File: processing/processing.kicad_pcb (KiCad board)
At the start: 2 copper layers, 26 parts, among them J1 HRO-TYPE-C-31-M-12, J2 Conn_01x03, J3 ICSP, SW1 SW_RESET, U1 CH340G, U2 ATmega328P-AU, Y1 12MHz, Y2 16MHz

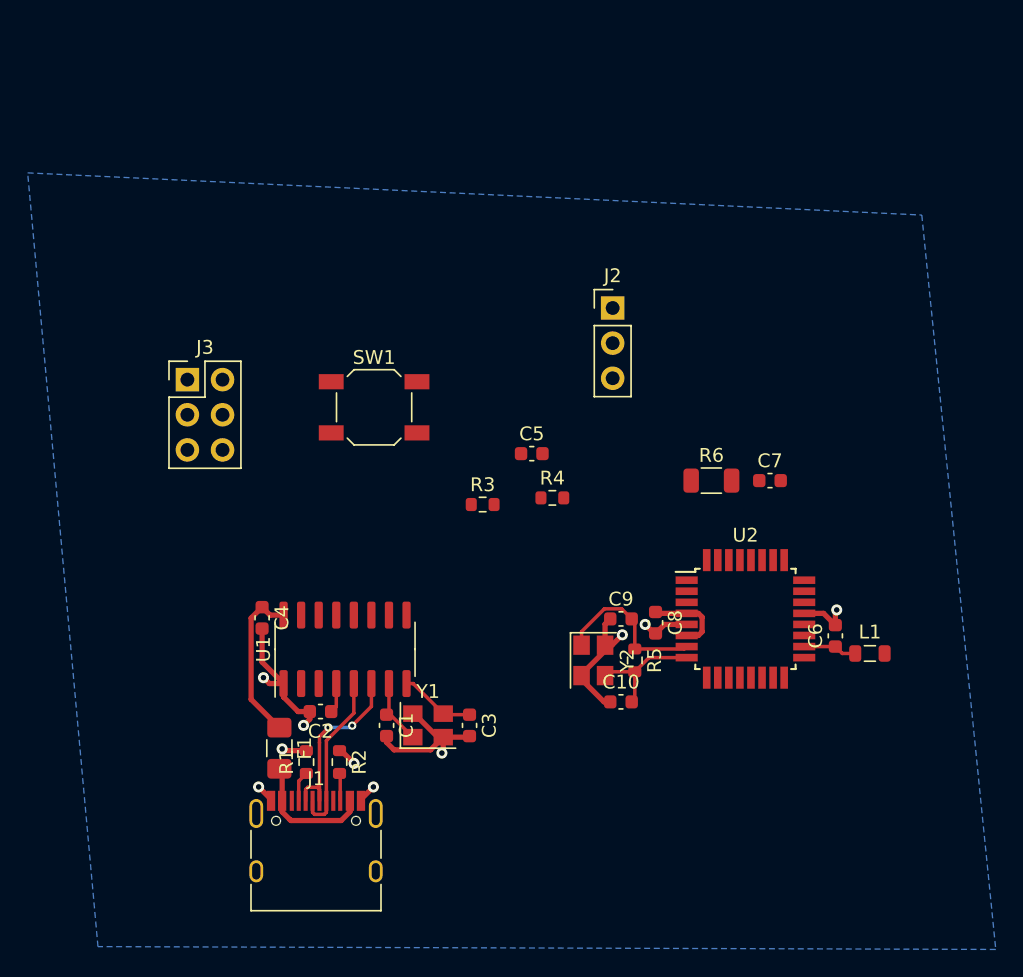
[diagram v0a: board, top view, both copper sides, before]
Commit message: finish the processing board
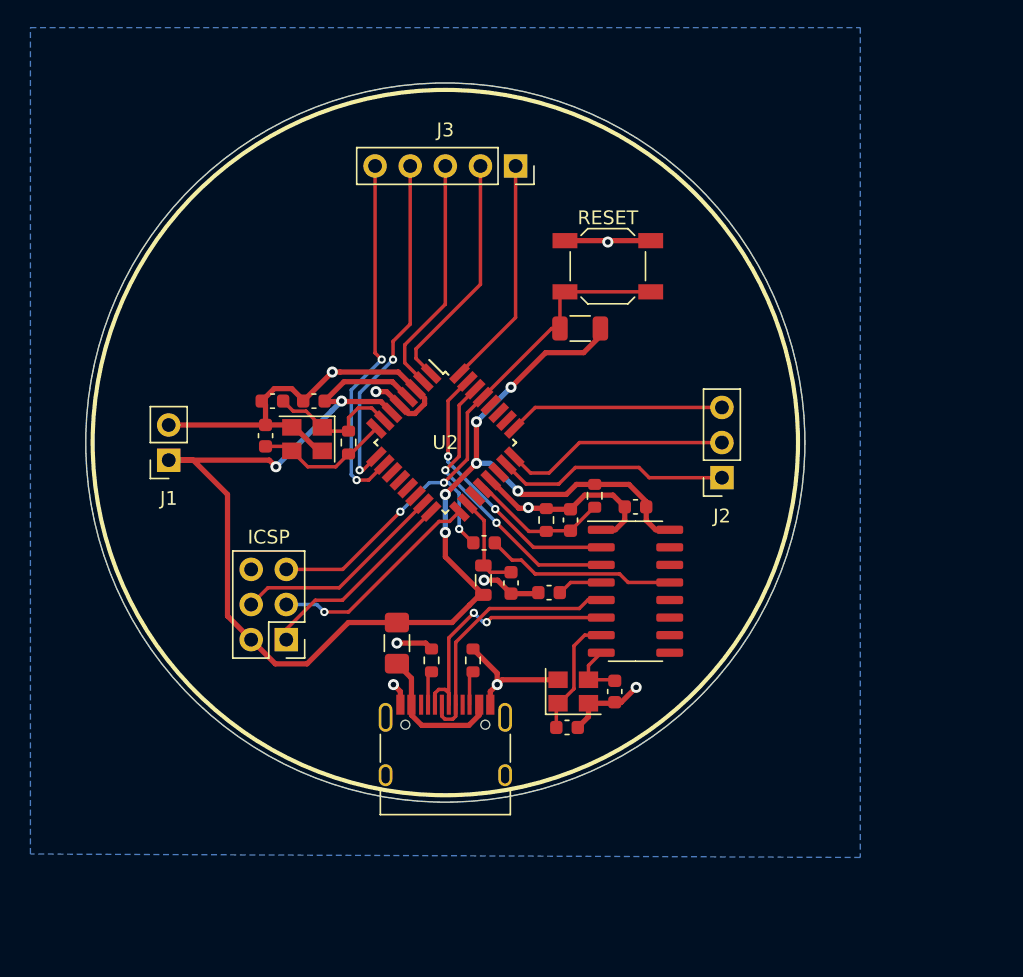
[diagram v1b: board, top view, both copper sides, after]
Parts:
- added J3: Conn_01x05, Connector_PinSocket_2.54mm:PinSocket_1x05_P2.54mm_Vertical, F.Cu at (155.4, 76.5)
- added J4: HRO-TYPE-C-31-M-12, Connector_USB:USB_C_Receptacle_HRO_TYPE-C-31-M-12, F.Cu at (150.3, 119.5)
- J1: value HRO-TYPE-C-31-M-12 -> Conn_01x02; footprint Connector_USB:USB_C_Receptacle_HRO_TYPE-C-31-M-12 -> Connector_PinSocket_2.54mm:PinSocket_1x02_P2.54mm_Vertical
- J2: footprint Connector_PinHeader_2.54mm:PinHeader_1x03_P2.54mm_Vertical -> Connector_PinSocket_2.54mm:PinSocket_1x03_P2.54mm_Vertical
- moved C10 32.1 mm to (137.3, 96.0), turned to 270 degrees
- moved J1 30.6 mm to (130.3, 97.8), turned to 180 degrees
- moved C9 29.7 mm to (137.8, 93.5)
- moved C8 29.4 mm to (140.8, 93.5), turned to 180 degrees
- moved L1 28.4 mm to (153.1, 106.5), turned to 270 degrees
- moved C4 28.2 mm to (164.1, 101.2), turned to 180 degrees
- moved Y2 26.2 mm to (140.3, 96.3), turned to 180 degrees
- moved R5 26.0 mm to (143.3, 96.5)
- moved U2 25.2 mm to (150.3, 96.5), turned to 315 degrees
- moved C6 23.8 mm to (155.1, 106.7), turned to 270 degrees
- moved U1 21.4 mm to (164.1, 107.3), turned to 0 degrees
- moved C7 21.2 mm to (153.2, 103.8)
- moved J5 20.1 mm to (138.8, 110.8), turned to 180 degrees
- moved SW1 19.7 mm to (162.1, 83.8), turned to 180 degrees
- moved C2 18.6 mm to (157.8, 107.4)
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- renumbered J3 to J5
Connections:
- J2 pad 3: A3 -> A2
- R1 pad 1: Net-(J1-PadA5) -> Net-(J4-PadA5)
- R2 pad 2: Net-(J1-PadB5) -> Net-(J4-PadB5)
- U1 pad 5: Net-(J1-PadA6) -> Net-(J4-PadA6)
- U1 pad 6: Net-(J1-PadA7) -> Net-(J4-PadA7)
- U2 pad 1: Net-(U2-Pad1) -> D2
- U2 pad 10: Net-(U2-Pad10) -> D5
- U2 pad 2: Net-(U2-Pad2) -> D3
- U2 pad 32: Net-(U2-Pad32) -> D1
- U2 pad 9: Net-(U2-Pad9) -> D4
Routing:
- net +5V: track 17.5 -> 106.7 mm, vias 0 -> 8
- net RESET: track 0.00 -> 43.4 mm, vias 0 -> 3
- net GND: track 44.9 -> 77.7 mm, vias 10 -> 9
- net D5: track 0.00 -> 26.4 mm, vias 0 -> 2
- net D4: track 0.00 -> 25.1 mm, vias 0 -> 2
- net RX: track 0.00 -> 20.9 mm, vias 0 -> 2
- net TX: track 0.00 -> 20.0 mm, vias 0 -> 2
- net Net-(J4-PadA7): track 0.00 -> 19.9 mm, vias 0 -> 2
- net Net-(J4-PadA6): track 0.00 -> 19.1 mm
- net D2: track 0.00 -> 17.4 mm
- net D3: track 0.00 -> 17.4 mm
- net A0: track 0.00 -> 17.0 mm
- net D1: track 0.00 -> 16.7 mm
- net A1: track 0.00 -> 16.4 mm
- net SCK: track 0.00 -> 15.8 mm, vias 0 -> 1
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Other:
- board outline added: 52 x 52 mm
- board text added: "RESET"
